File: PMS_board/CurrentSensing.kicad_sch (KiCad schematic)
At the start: 7 parts, among them U2 LM324DR, U20 MCP3204T-CI/ST

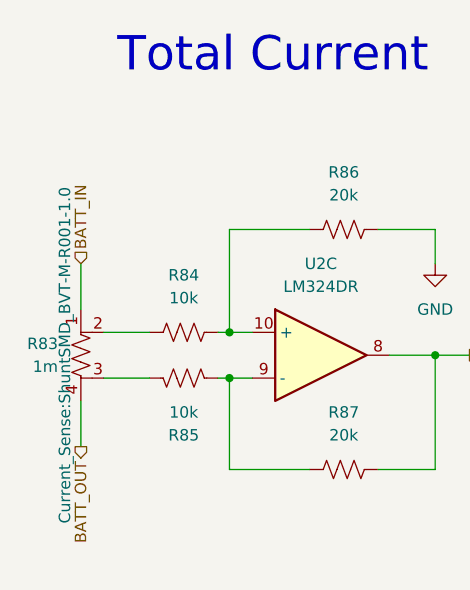
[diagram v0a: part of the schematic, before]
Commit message: Revert "Add changes from Review"
This reverts commit e7e7edd03615e33a608a50c27cdb501654904b7f.
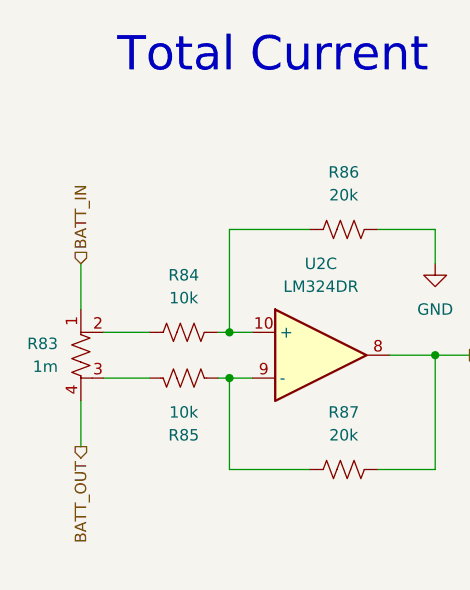
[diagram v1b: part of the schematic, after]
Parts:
- R83: footprint Current_Sense:ShuntSMD_BVT-M-R001-1.0 -> Footprints:ShuntSMD_BVT-M-R001-1.0
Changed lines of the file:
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@@
 			)
 		)
-		(property "Footprint" "Current_Sense:ShuntSMD_BVT-M-R001-1.0"
+		(property "Footprint" "Footprints:ShuntSMD_BVT-M-R001-1.0"
 			(at 79.502 102.87 90)
+			(hide yes)
 			(show_name no)
 			(do_not_autoplace no)

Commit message: Add changes from Review
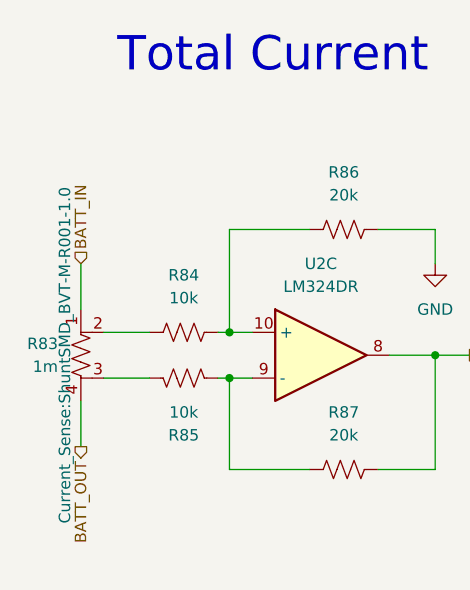
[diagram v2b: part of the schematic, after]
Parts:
- R83: footprint Footprints:ShuntSMD_BVT-M-R001-1.0 -> Current_Sense:ShuntSMD_BVT-M-R001-1.0
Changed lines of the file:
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@@
 			)
 		)
-		(property "Footprint" "Footprints:ShuntSMD_BVT-M-R001-1.0"
+		(property "Footprint" "Current_Sense:ShuntSMD_BVT-M-R001-1.0"
 			(at 79.502 102.87 90)
-			(hide yes)
 			(show_name no)
 			(do_not_autoplace no)
